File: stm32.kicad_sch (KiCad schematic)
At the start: 7 parts, among them U3 STM32G431RBT6

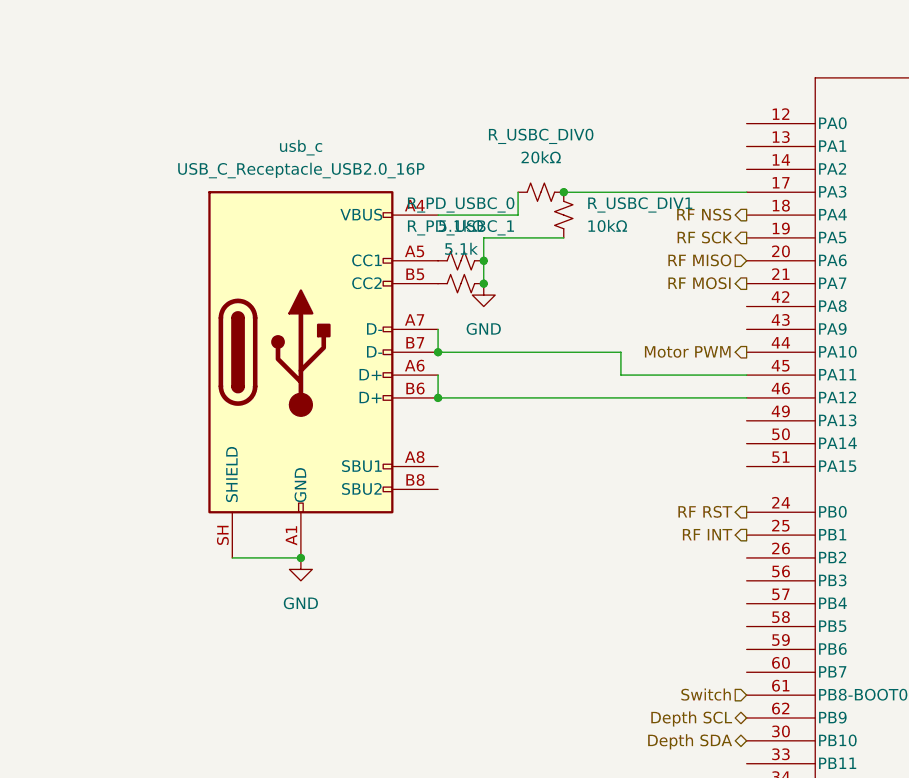
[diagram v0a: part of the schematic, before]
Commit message: Checkpoint
Checkpoint, pre battery telemetry, pre new stm
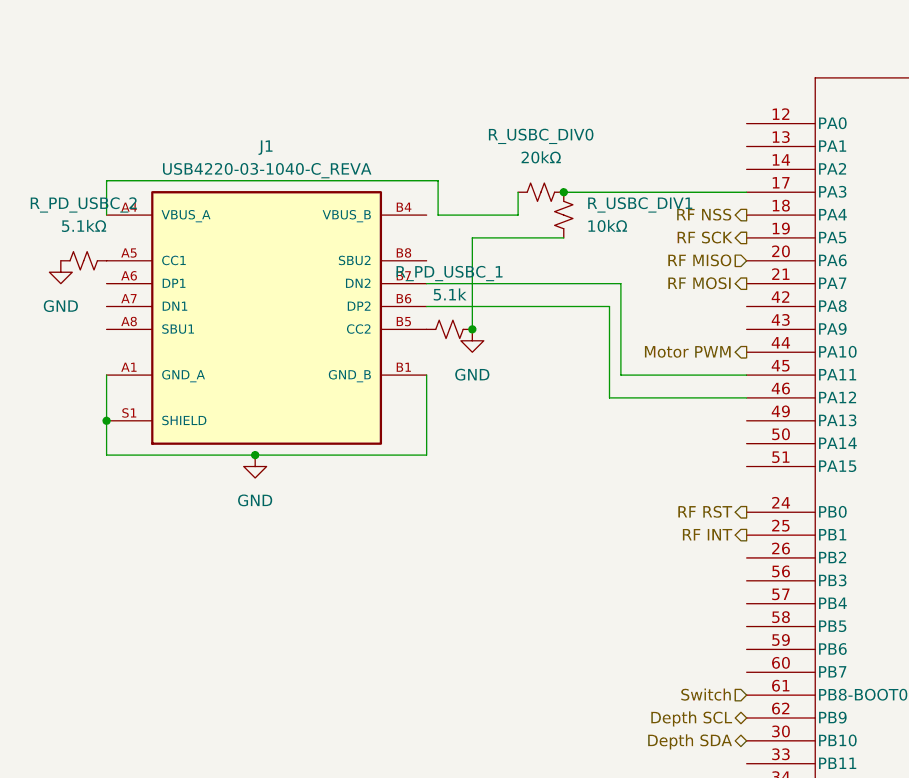
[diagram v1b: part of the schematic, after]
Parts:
- removed R_PD_USBC_0: 5.1kΩ, Resistor_SMD:R_0603_1608Metric, symbol Device:R_Small_US
- removed usb_c: USB_C_Receptacle_USB2.0_16P, symbol Connector:USB_C_Receptacle_USB2.0_16P
- added J1: USB4220-03-1040-C_REVA, usbc:GCT_USB4220-03-1040-C_REVA, symbol usbc:USB4220-03-1040-C_REVA
- added R_PD_USBC_2: 5.1kΩ, Resistor_SMD:R_0603_1608Metric, symbol Device:R_Small_US
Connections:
- net GND: now also J1.A1 (GND_A), J1.A12 (GND_A), J1.B1 (GND_B), J1.B12 (GND_A), J1.S1 (SHIELD), J1.S2 (SHIELD), J1.S3 (SHIELD), J1.S4 (SHIELD), R_PD_USBC_2.1
- net at R_PD_USBC_1.1: now also J1.B5 (CC2)
- net VBUS_A: now reaches R_USBC_DIV0.1
- net VBUS_A: now also J1.A4 (VBUS_A), J1.A9 (VBUS_A)
- net at U3.46 (PA12): now also J1.B6 (DP2)
- net at U3.45 (PA11): now also J1.B7 (DN2)
- new net: J1.A5 (CC1), R_PD_USBC_2.2
- new net VBUS_B: J1.B4 (VBUS_B), J1.B9 (VBUS_B)

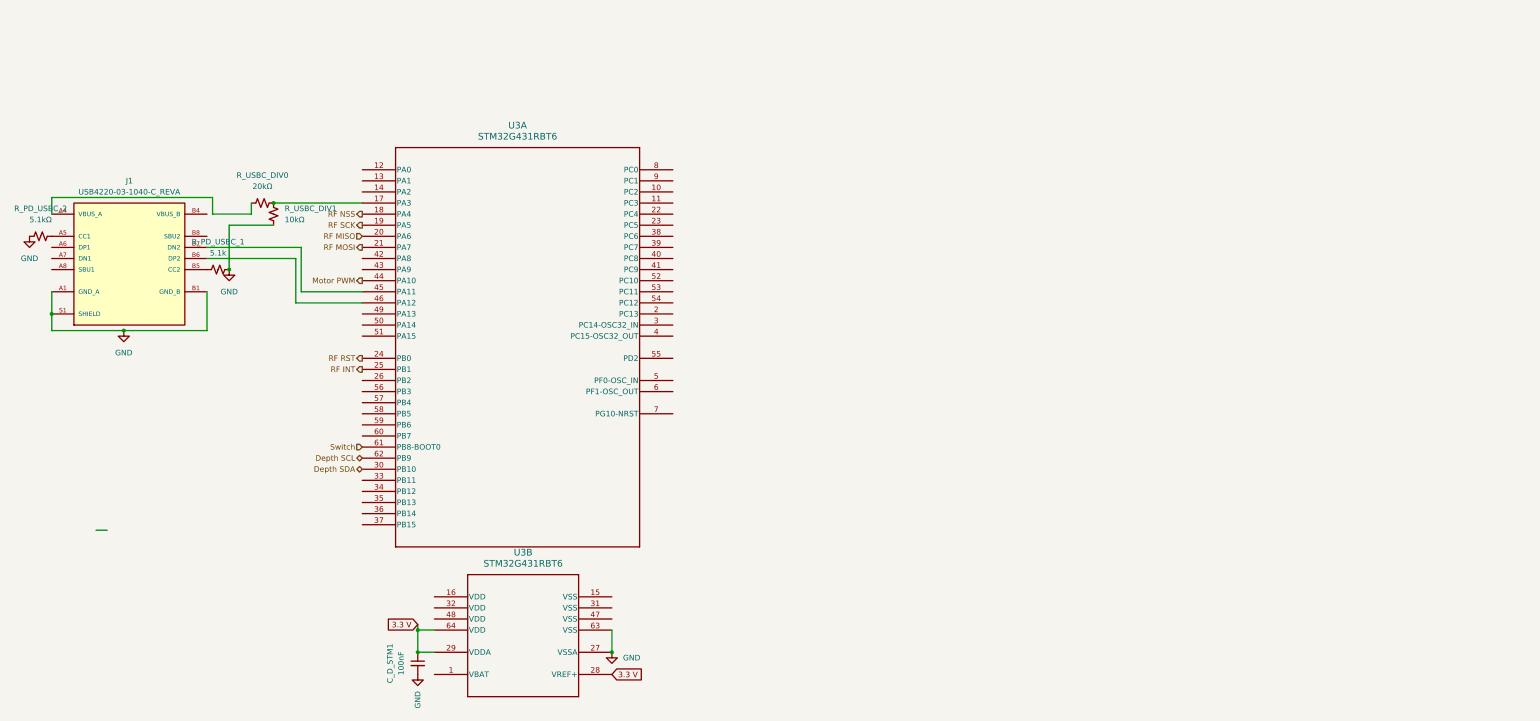
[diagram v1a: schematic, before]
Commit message: Update
Update
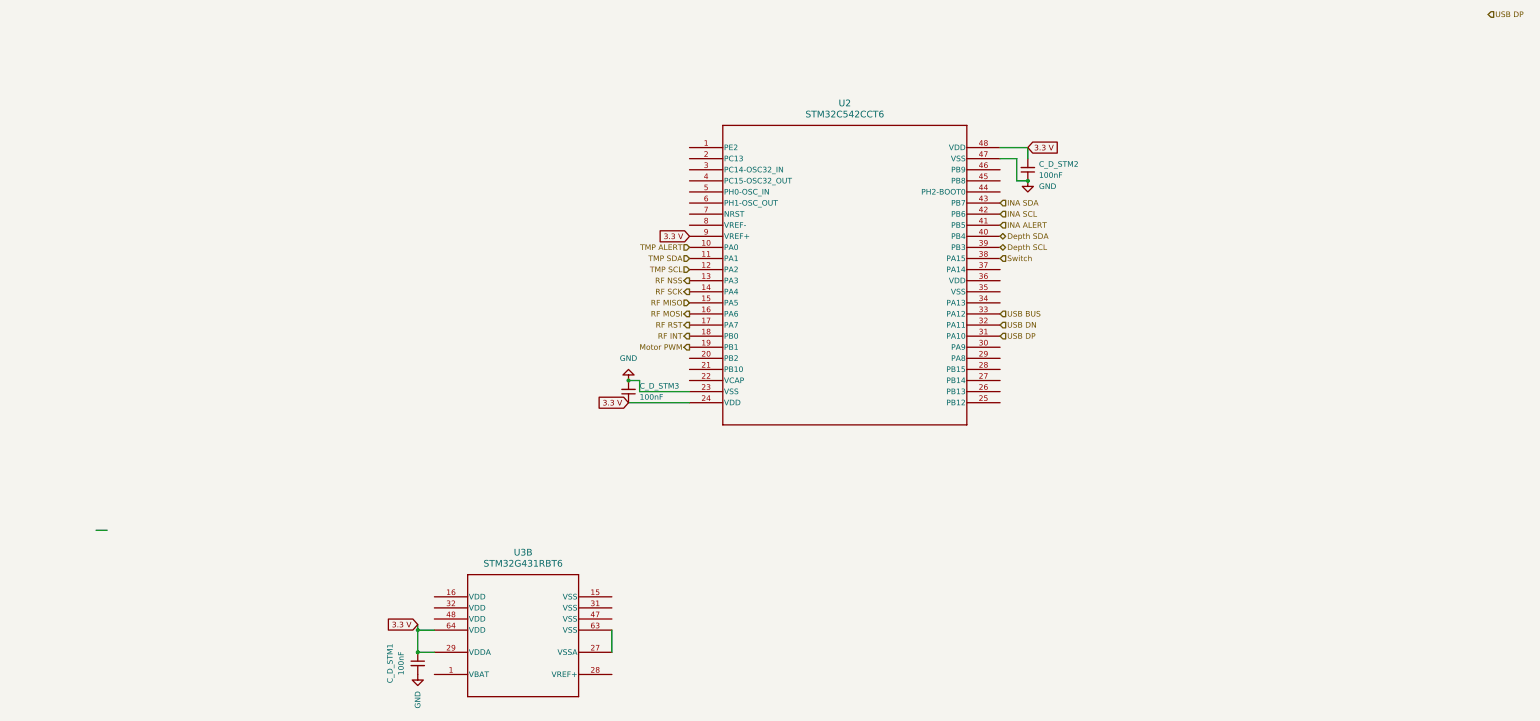
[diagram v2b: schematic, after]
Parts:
- removed J1: USB4220-03-1040-C_REVA, usbc:GCT_USB4220-03-1040-C_REVA, symbol usbc:USB4220-03-1040-C_REVA
- removed R_PD_USBC_1: 5.1k, Resistor_SMD:R_0603_1608Metric, symbol Device:R_Small_US
- removed R_PD_USBC_2: 5.1kΩ, Resistor_SMD:R_0603_1608Metric, symbol Device:R_Small_US
- removed R_USBC_DIV0: 20kΩ, Resistor_SMD:R_0603_1608Metric, symbol Device:R_Small_US
- removed R_USBC_DIV1: 10kΩ, Resistor_SMD:R_0603_1608Metric, symbol Device:R_Small_US
- removed unit 1 of U3
- added C_D_STM2, C_D_STM3: 100nF, Capacitor_SMD:C_0603_1608Metric, symbol Device:C_Small
- added U2: STM32C542CCT6, LQFP48-7X7, symbol STM32:STM32C542CCT6
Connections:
- net 3.3 V: now also C_D_STM2.2, C_D_STM3.1, U2.24 (VDD), U2.48 (VDD), U2.9 (VREF+); no longer U3.28 (VREF+)
- net Depth SCL: now also U2.39 (PB3)
- net Depth SDA: now also U2.40 (PB4)
- net GND: now also C_D_STM2.1, C_D_STM3.2, U2.23 (VSS), U2.47 (VSS); no longer U3.27 (VSSA), U3.63 (VSS)
- net Motor PWM: now also U2.19 (PB1)
- net RF INT: now also U2.18 (PB0)
- net RF MISO: now also U2.15 (PA5)
- net RF MOSI: now also U2.16 (PA6)
- net RF NSS: now also U2.13 (PA3)
- net RF RST: now also U2.17 (PA7)
- net RF SCK: now also U2.14 (PA4)
- net Switch: now also U2.38 (PA15)
- new net: U3.27 (VSSA), U3.63 (VSS)
- new net INA ALERT: U2.41 (PB5)
- new net INA SCL: U2.42 (PB6)
- new net INA SDA: U2.43 (PB7)
- new net TMP ALERT: U2.10 (PA0)
- new net TMP SCL: U2.12 (PA2)
- new net TMP SDA: U2.11 (PA1)
- new net USB BUS: U2.33 (PA12)
- new net USB DN: U2.32 (PA11)
- new net USB DP: U2.31 (PA10)
